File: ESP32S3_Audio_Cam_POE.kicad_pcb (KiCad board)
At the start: 4 copper layers, 56 parts, among them J1 USB-C, U1 USBLC6-2SC6, U2 TLV62568DBVR, U3 ESP32-S3R8, Y1 40MHz, Y2 32.768KHz

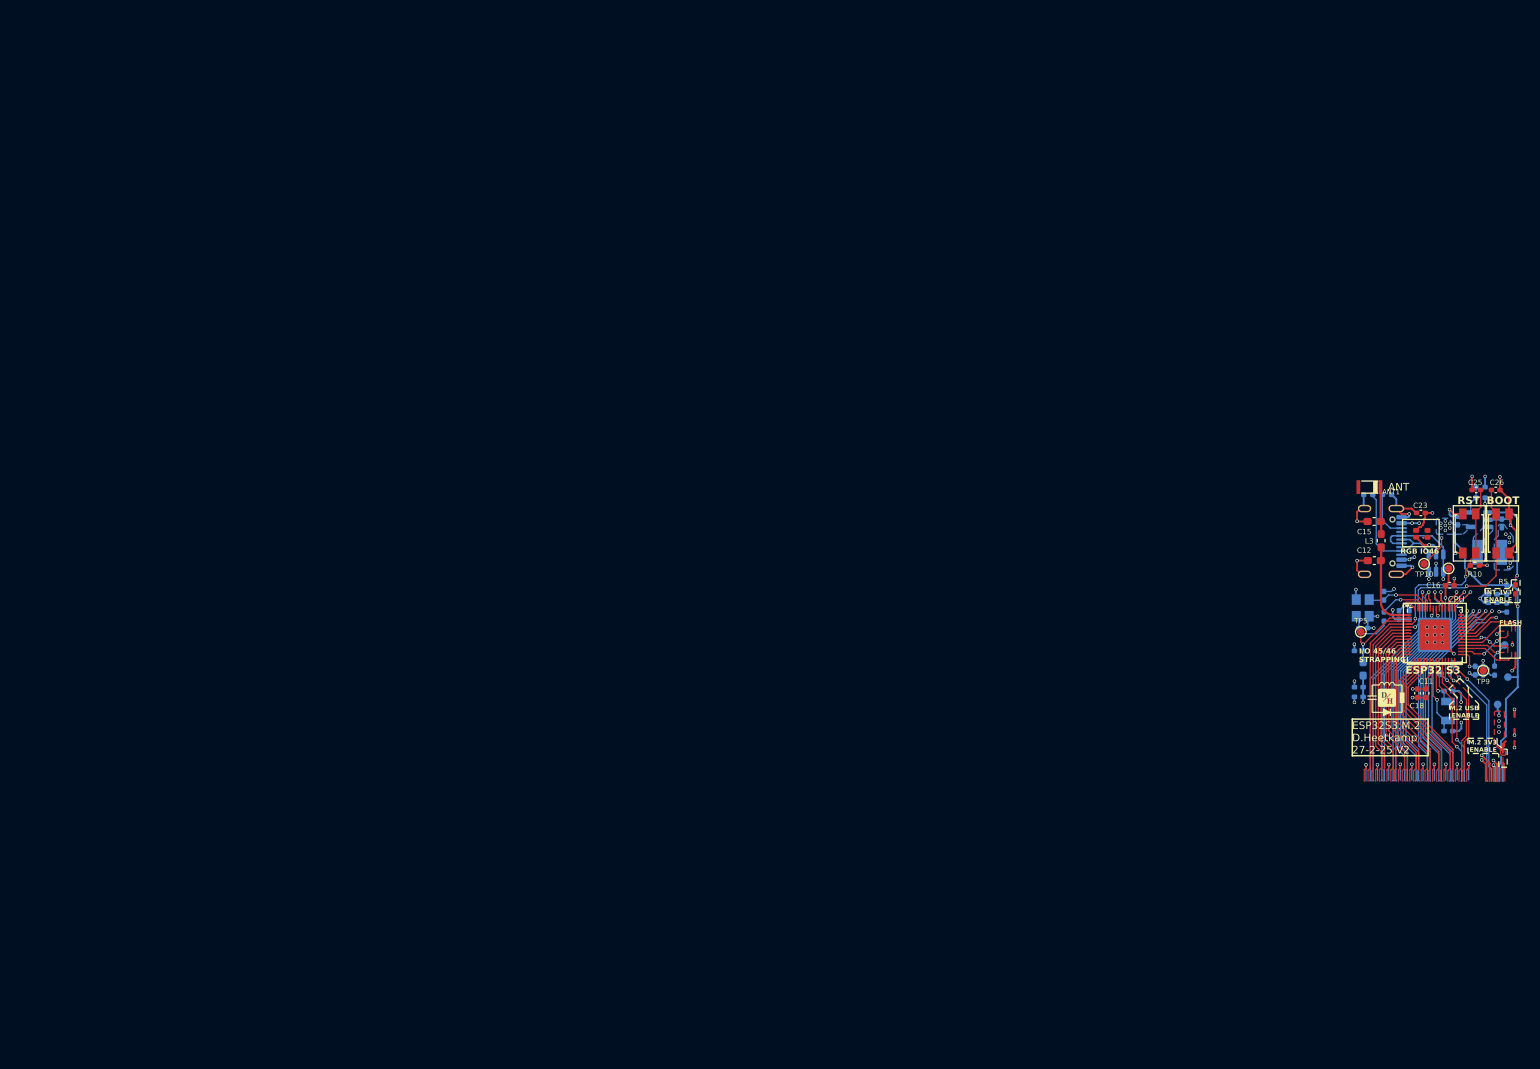
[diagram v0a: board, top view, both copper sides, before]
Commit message: Draft commit, needs routing, schematic is probably mostly OK. Footprints are roughly located.
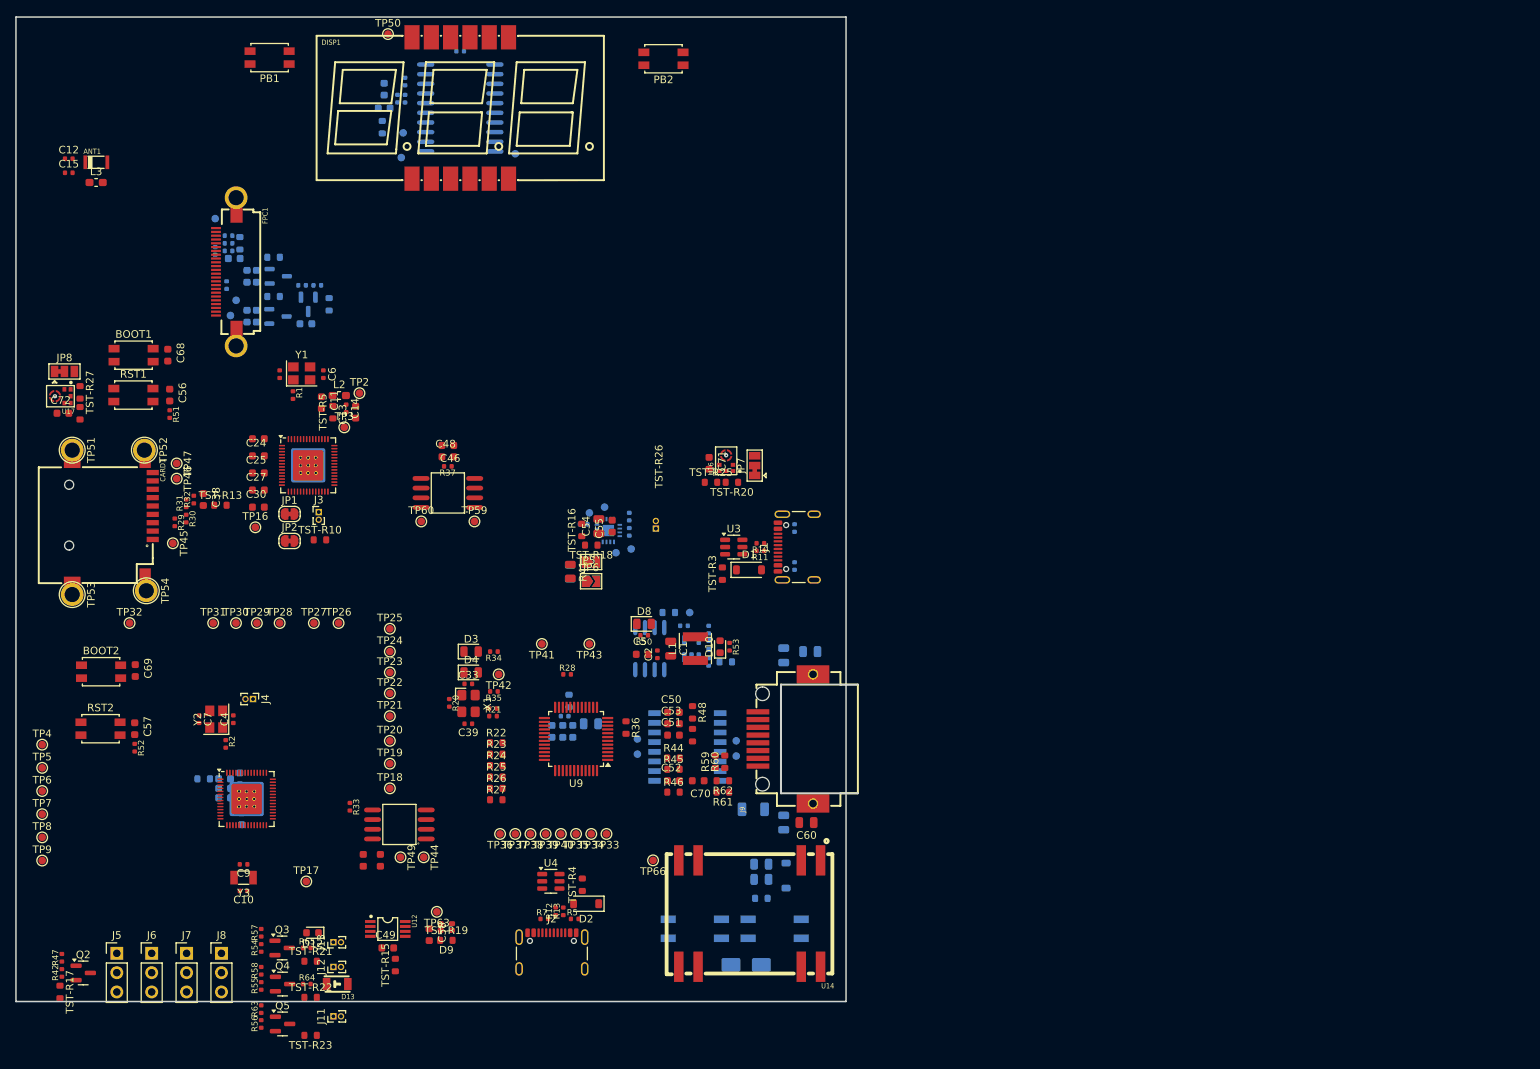
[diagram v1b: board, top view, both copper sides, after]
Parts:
- removed G***: LOGO, LOGO
- removed LED1: WS2812C-2020-V1, PCM_JLCPCB:LED-SMD_4P-L1.6-W1.5_XL-1615RGBC-WS2812B
- removed TP10: TestPoint, TestPoint:TestPoint_Pad_D1.0mm
- added BOOT2: SW_BOOT, Button_Switch_SMD:SW_SPST_EVQP2, F.Cu at (53.4, 117.4)
- added C1: 4.7uF, PCM_JLCPCB:C_0805, F.Cu at (128.4, 114.4)
- added C2: 1nF, PCM_JLCPCB:C_0402, F.Cu at (126.6, 115.2)
- added C27: 100nF, PCM_JLCPCB:C_0603, F.Cu at (74.1, 93.5)
- added C28: 100nF, PCM_JLCPCB:C_0603, B.Cu at (71.7, 131.5)
- added C29: 100nF, PCM_JLCPCB:C_0603, B.Cu at (71.9, 136.8)
- added C3: 10pF, PCM_JLCPCB:C_0402, F.Cu at (76.9, 78.3)
- added C30: 100nF, PCM_JLCPCB:C_0603, F.Cu at (74.1, 95.8)
- added C31: 100nF, PCM_JLCPCB:C_0603, B.Cu at (69.7, 131.5)
- added C32: 100nF, PCM_JLCPCB:C_0603, B.Cu at (69.7, 132.8)
- added C33: 10pF, PCM_JLCPCB:C_0402, F.Cu at (101.8, 119.0)
- added C34: 10pF, PCM_JLCPCB:C_0402, F.Cu at (105.0, 122.3)
- added C35: 100nF, PCM_JLCPCB:C_0603, B.Cu at (114.2, 125.3)
- added C36: 10uF, PCM_JLCPCB:C_0805, B.Cu at (117.9, 124.3)
- added C37: 100nF, PCM_JLCPCB:C_0603, B.Cu at (112.8, 125.3)
- added C38: 100nF, PCM_JLCPCB:C_0603, F.Cu at (66.9, 94.8)
- added C39: 10nF, PCM_JLCPCB:C_0402, F.Cu at (101.8, 124.3)
- added C4: 10pF, PCM_JLCPCB:C_0402, F.Cu at (70.8, 123.7)
- added C40: 4.7uF, PCM_JLCPCB:C_0603, B.Cu at (115.5, 125.3)
- added C41: 100nF, PCM_JLCPCB:C_0603, F.Cu at (90.2, 142.3)
- added C42: 1uF, PCM_JLCPCB:C_0603, F.Cu at (87.9, 142.3)
- added C43: 1uF, PCM_JLCPCB:C_0603, B.Cu at (90.7, 40.8)
- added C44: 100nF, PCM_JLCPCB:C_0603, B.Cu at (90.7, 43.3)
- added C45: 100pF, PCM_JLCPCB:C_0402, B.Cu at (100.7, 35.8)
- added C46: 100nF, PCM_JLCPCB:C_0603, F.Cu at (99.1, 87.7)
- added C47: 100pF, PCM_JLCPCB:C_0402, B.Cu at (93.4, 39.8)
- added C48: 1uF, PCM_JLCPCB:C_0603, F.Cu at (99.1, 89.2)
- added C49: 100nF, PCM_JLCPCB:C_0603, F.Cu at (91.2, 153.8)
- added C5: 100nF, PCM_JLCPCB:C_0603, F.Cu at (124.6, 115.2)
- added C50: 6.8nF, PCM_JLCPCB:C_0603, F.Cu at (128.8, 122.8)
- added C51: 6.8nF, PCM_JLCPCB:C_0603, F.Cu at (128.8, 125.8)
- added C52: 220nF, PCM_JLCPCB:C_0603, F.Cu at (128.8, 131.8)
- added C53: 220nF, PCM_JLCPCB:C_0603, F.Cu at (128.8, 124.3)
- added C54: 10uF, PCM_JLCPCB:C_0805, F.Cu at (118.9, 98.3)
- added C55: 100nF, PCM_JLCPCB:C_0603, F.Cu at (120.7, 98.3)
- added C56: 100nF, PCM_JLCPCB:C_0603, F.Cu at (62.5, 81.0)
- added C57: 100nF, PCM_JLCPCB:C_0603, F.Cu at (57.9, 124.9)
- added C58: 100nF, PCM_JLCPCB:C_0603, F.Cu at (96.6, 152.0)
- added C59: 100nF, PCM_JLCPCB:C_0805, B.Cu at (143.3, 137.3)
- added C60: 100nF, PCM_JLCPCB:C_0805, F.Cu at (146.3, 137.3)
- added C61: 10uF, PCM_JLCPCB:C_0805, B.Cu at (140.3, 144.8)
- added C62: 100nF, PCM_JLCPCB:C_0805, B.Cu at (146.8, 114.8)
- added C63: 100nF, PCM_JLCPCB:C_0805, B.Cu at (143.3, 115.3)
- added C64: 22uF, PCM_JLCPCB:C_0805, B.Cu at (140.3, 142.8)
- added C65: 1nF, PCM_JLCPCB:C_1206, B.Cu at (139.3, 135.5)
- added C66: 220pF, PCM_JLCPCB:C_0402, B.Cu at (122.9, 99.0)
- added C67: 220pF, PCM_JLCPCB:C_0402, B.Cu at (122.9, 97.0)
- added C68: 100nF, PCM_JLCPCB:C_0603, F.Cu at (62.2, 75.8)
- added C69: 100nF, PCM_JLCPCB:C_0603, F.Cu at (57.9, 117.3)
- added C70: 100nF, PCM_JLCPCB:C_0603, F.Cu at (132.0, 131.8)
- added C71: 100nF, PCM_JLCPCB:C_0603, F.Cu at (133.4, 90.0)
- added C72: 100nF, PCM_JLCPCB:C_0603, F.Cu at (48.4, 83.4)
- added CARD1: TF PUSH, JLCPCB:TF-PUSH-SD-CARD_C393941, F.Cu at (54.9, 97.8)
- added D10: Red, PCM_JLCPCB:D_0603, F.Cu at (134.9, 114.2)
- added D11: 1N4148W, PCM_JLCPCB:D_SOD-123, B.Cu at (143.6, 144.3)
- added D12: White, PCM_JLCPCB:D_0603, F.Cu at (81.3, 151.8)
- added D13: IR, JLCPCB:IR-LED_C131280, F.Cu at (84.5, 158.5)
- added D3: Yellow, PCM_JLCPCB:D_0805, F.Cu at (102.1, 114.8)
- added D4: Green, PCM_JLCPCB:D_0805, F.Cu at (102.1, 117.5)
- added D5: MB6S, JLCPCB:MB6S-C82584, B.Cu at (131.6, 151.3)
- added D6: MB6S, JLCPCB:MB6S-C82584, B.Cu at (142.1, 151.3)
- added D7: SMAJ58A, PCM_JLCPCB:D_SMA, B.Cu at (138.3, 156.0)
- added D8: Green, PCM_JLCPCB:D_0805, F.Cu at (124.9, 111.2)
- added D9: WS2812B, PCM_JLCPCB:LED-SMD_4P-L1.6-W1.5_XL-1615RGBC-WS2812B, F.Cu at (98.9, 151.0)
- added DISP1: SLS0563DRA1GD, JLCPCB:3x7-seg_LED-RED_C2913084, F.Cu at (100.7, 43.3)
- added FPC1: AFC01-S24FCC-00, JLCPCB:OV2640_connector_AFC01-S24FCC-00, F.Cu at (69.9, 64.8)
- added J10: Conn_01x02, Connector_PinHeader_1.00mm:PinHeader_1x02_P1.00mm_Vertical, B.Cu at (126.4, 98.6)
- added J11: Conn_01x02, Connector_PinHeader_1.00mm:PinHeader_1x02_P1.00mm_Vertical, F.Cu at (84.0, 162.8)
- added J12: Conn_01x02, Connector_PinHeader_1.00mm:PinHeader_1x02_P1.00mm_Vertical, F.Cu at (84.0, 156.3)
- added J13: Conn_01x02, Connector_PinHeader_1.00mm:PinHeader_1x02_P1.00mm_Vertical, F.Cu at (84.0, 153.0)
- added J2: USB-C, Connector_USB:USB_C_Receptacle_GCT_USB4105-xx-A_16P_TopMnt_Horizontal, F.Cu at (112.8, 155.5)
- added J3: Conn_01x02, Connector_PinHeader_1.00mm:PinHeader_1x02_P1.00mm_Vertical, F.Cu at (82.1, 96.4)
- added J4: Conn_01x02, Connector_PinHeader_1.00mm:PinHeader_1x02_P1.00mm_Vertical, F.Cu at (73.4, 121.0)
- added J5: Conn_01x03, Connector_PinHeader_2.54mm:PinHeader_1x03_P2.54mm_Vertical, F.Cu at (55.5, 154.5)
- added J6: Conn_01x03, Connector_PinHeader_2.54mm:PinHeader_1x03_P2.54mm_Vertical, F.Cu at (60.1, 154.5)
- added J7: Conn_01x03, Connector_PinHeader_2.54mm:PinHeader_1x03_P2.54mm_Vertical, F.Cu at (64.7, 154.5)
- added J8: Conn_01x03, Connector_PinHeader_2.54mm:PinHeader_1x03_P2.54mm_Vertical, F.Cu at (69.3, 154.5)
- added J9: HC-RJ45-055-4_8P8C_Shielded, JLCPCB:HC-RJ45-055-4_C3000211, F.Cu at (143.5, 126.3)
- added JP1: Jumper_2_Small_Bridged, Jumper:SolderJumper-2_P1.3mm_Bridged_RoundedPad1.0x1.5mm, F.Cu at (78.2, 96.7)
- added JP2: Jumper_2_Small_Bridged, Jumper:SolderJumper-2_P1.3mm_Bridged_RoundedPad1.0x1.5mm, F.Cu at (78.2, 100.2)
- added JP3: SolderJumper_2_Open, Jumper:SolderJumper-2_P1.3mm_Open_TrianglePad1.0x1.5mm, B.Cu at (117.9, 105.5)
- added JP4: SolderJumper_2_Open, Jumper:SolderJumper-2_P1.3mm_Open_TrianglePad1.0x1.5mm, B.Cu at (117.9, 103.0)
- added JP5: SolderJumper_2_Open, Jumper:SolderJumper-2_P1.3mm_Open_TrianglePad1.0x1.5mm, F.Cu at (117.9, 103.0)
- added JP6: SolderJumper_2_Open, Jumper:SolderJumper-2_P1.3mm_Open_TrianglePad1.0x1.5mm, F.Cu at (117.9, 105.5)
- added JP7: SolderJumper_3_Bridged12, Jumper:SolderJumper-3_P1.3mm_Bridged12_Pad1.0x1.5mm, F.Cu at (139.4, 90.3)
- added JP8: SolderJumper_3_Bridged12, Jumper:SolderJumper-3_P1.3mm_Bridged12_Pad1.0x1.5mm, F.Cu at (48.6, 77.9)
- added L4: 3.9nH,300mA, PCM_JLCPCB:L_0402, B.Cu at (114.4, 123.3)
- added PB1: SW_RST, Button_Switch_SMD:SW_SPST_EVQP2, F.Cu at (75.6, 36.6)
- added PB2: SW_RST, Button_Switch_SMD:SW_SPST_EVQP2, F.Cu at (127.4, 36.8)
- added Q1: AO3401A, PCM_JLCPCB:Q_SOT-23, B.Cu at (80.7, 69.1)
- added Q2: AO3401A, PCM_JLCPCB:Q_SOT-23, F.Cu at (51.1, 157.1)
- added Q3: AO3401A, PCM_JLCPCB:Q_SOT-23, F.Cu at (77.3, 153.8)
- added Q4: AO3401A, PCM_JLCPCB:Q_SOT-23, F.Cu at (77.3, 158.5)
- added Q5: AO3401A, PCM_JLCPCB:Q_SOT-23, F.Cu at (77.3, 163.8)
- added R13: 33Ω, PCM_JLCPCB:R_0402, F.Cu at (114.3, 149.0)
- added R14: 10MΩ, PCM_JLCPCB:R_0402, B.Cu at (81.9, 66.6)
- added R15: 1MΩ, PCM_JLCPCB:R_0402, B.Cu at (79.9, 66.6)
- added R16: 10kΩ, PCM_JLCPCB:R_0402, B.Cu at (70.2, 60.1)
- added R17: 10kΩ, PCM_JLCPCB:R_0402, B.Cu at (70.2, 61.1)
- added R18: 10kΩ, PCM_JLCPCB:R_0402, B.Cu at (70.2, 62.1)
- added R19: 10kΩ, PCM_JLCPCB:R_0402, B.Cu at (68.5, 62.1)
- added R20: 1MΩ, PCM_JLCPCB:R_0402, F.Cu at (99.3, 121.5)
- added R21: 0Ω, PCM_JLCPCB:R_0402, F.Cu at (105.0, 123.3)
- added R22: 20Ω, PCM_JLCPCB:R_0603, F.Cu at (105.4, 126.8)
- added R23: 20Ω, PCM_JLCPCB:R_0603, F.Cu at (105.4, 128.3)
- added R24: 20Ω, PCM_JLCPCB:R_0603, F.Cu at (105.4, 129.8)
- added R25: 20Ω, PCM_JLCPCB:R_0603, F.Cu at (105.4, 131.3)
- added R26: 20Ω, PCM_JLCPCB:R_0603, F.Cu at (105.4, 132.8)
- added R27: 20Ω, PCM_JLCPCB:R_0603, F.Cu at (105.4, 134.3)
- added R28: 10kΩ, PCM_JLCPCB:R_0402, F.Cu at (114.8, 117.8)
- added R29: 10kΩ, PCM_JLCPCB:R_0402, F.Cu at (63.1, 97.8)
- added R3: 22Ω, PCM_JLCPCB:R_0402, B.Cu at (130.1, 111.4)
- added R30: 10kΩ, PCM_JLCPCB:R_0402, F.Cu at (64.6, 97.3)
- added R31: 10kΩ, PCM_JLCPCB:R_0402, F.Cu at (64.6, 95.3)
- added R32: 10kΩ, PCM_JLCPCB:R_0402, F.Cu at (65.6, 94.8)
- added R33: 100kΩ, PCM_JLCPCB:R_0402, F.Cu at (86.2, 135.2)
- added R34: 680Ω, PCM_JLCPCB:R_0402, F.Cu at (105.1, 114.8)
- added R35: 680Ω, PCM_JLCPCB:R_0402, F.Cu at (105.1, 120.0)
- added R36: 12kΩ, PCM_JLCPCB:R_0603, F.Cu at (122.5, 124.8)
- added R37: 100kΩ, PCM_JLCPCB:R_0402, F.Cu at (99.1, 90.4)
- added R38: 10kΩ, PCM_JLCPCB:R_0402, B.Cu at (92.4, 42.0)
- added R39: 10kΩ, PCM_JLCPCB:R_0402, B.Cu at (93.4, 42.0)
- added R4: 5.1kΩ, PCM_JLCPCB:R_0402, B.Cu at (144.7, 98.5)
- added R40: 100kΩ, PCM_JLCPCB:R_0805, B.Cu at (115.2, 104.3)
- added R41: 100kΩ, PCM_JLCPCB:R_0805, F.Cu at (115.2, 104.3)
- added R42: 10MΩ, PCM_JLCPCB:R_0402, F.Cu at (48.3, 157.1)
- added R43: 1MΩ, PCM_JLCPCB:R_0402, B.Cu at (116.9, 98.0)
- added R44: 47Ω, PCM_JLCPCB:R_0603, F.Cu at (128.8, 128.8)
- added R45: 47Ω, PCM_JLCPCB:R_0603, F.Cu at (128.8, 130.3)
- added R46: 47Ω, PCM_JLCPCB:R_0603, F.Cu at (128.8, 133.3)
- added R47: 1MΩ, PCM_JLCPCB:R_0402, F.Cu at (48.3, 155.1)
- added R48: 82Ω, PCM_JLCPCB:R_0603, F.Cu at (131.3, 122.8)
- added R49: 82Ω, PCM_JLCPCB:R_0603, F.Cu at (131.3, 125.8)
- added R50: 10kΩ, PCM_JLCPCB:R_0402, F.Cu at (124.9, 112.7)
- added R51: 10kΩ, PCM_JLCPCB:R_0402, F.Cu at (62.5, 83.5)
- added R52: 10kΩ, PCM_JLCPCB:R_0402, F.Cu at (57.9, 127.4)
- added R53: 10kΩ, PCM_JLCPCB:R_0402, F.Cu at (136.1, 114.2)
- added R54: 10MΩ, PCM_JLCPCB:R_0402, F.Cu at (74.5, 153.8)
- added R55: 10MΩ, PCM_JLCPCB:R_0402, F.Cu at (74.5, 158.8)
- added R56: 10MΩ, PCM_JLCPCB:R_0402, F.Cu at (74.5, 163.8)
- added R57: 1MΩ, PCM_JLCPCB:R_0402, F.Cu at (74.5, 151.8)
- added R58: 1MΩ, PCM_JLCPCB:R_0402, F.Cu at (74.5, 156.8)
- added R59: 75Ω, PCM_JLCPCB:R_0603, F.Cu at (134.3, 129.3)
- added R60: 75Ω, PCM_JLCPCB:R_0603, F.Cu at (135.5, 129.3)
- added R61: 75Ω, PCM_JLCPCB:R_0603, F.Cu at (135.3, 133.3)
- added R62: 75Ω, PCM_JLCPCB:R_0603, F.Cu at (135.3, 131.8)
- added R63: 1MΩ, PCM_JLCPCB:R_0402, F.Cu at (74.5, 161.8)
- added R64: 10kΩ, PCM_JLCPCB:R_0402, F.Cu at (80.5, 158.5)
- added R65: 10kΩ, PCM_JLCPCB:R_0402, F.Cu at (80.5, 153.8)
- added RST2: SW_RST, Button_Switch_SMD:SW_SPST_EVQP2, F.Cu at (53.4, 124.9)
- added T1: H1102NLT, JLCPCB:H1102NLT_C18584, B.Cu at (130.6, 127.3)
- added TP11: TestPoint, TestPoint:TestPoint_Pad_D1.0mm, B.Cu at (68.5, 57.8)
- added TP12: TestPoint, TestPoint:TestPoint_Pad_D1.0mm, B.Cu at (71.2, 68.6)
- added TP13: TestPoint, TestPoint:TestPoint_Pad_D1.0mm, B.Cu at (70.5, 70.6)
- added TP14: TestPoint, TestPoint:TestPoint_Plated_Hole_D2.0mm, B.Cu at (71.2, 55.1)
- added TP15: TestPoint, TestPoint:TestPoint_Plated_Hole_D2.0mm, B.Cu at (71.2, 74.6)
- added TP16: TestPoint, TestPoint:TestPoint_Pad_D1.0mm, F.Cu at (73.7, 98.4)
- added TP17: TestPoint, TestPoint:TestPoint_Pad_D1.0mm, F.Cu at (80.4, 145.0)
- added TP18: TestPoint, TestPoint:TestPoint_Pad_D1.0mm, F.Cu at (91.4, 132.8)
- added TP19: TestPoint, TestPoint:TestPoint_Pad_D1.0mm, F.Cu at (91.4, 129.5)
- added TP20: TestPoint, TestPoint:TestPoint_Pad_D1.0mm, F.Cu at (91.4, 126.5)
- added TP21: TestPoint, TestPoint:TestPoint_Pad_D1.0mm, F.Cu at (91.4, 123.3)
- added TP22: TestPoint, TestPoint:TestPoint_Pad_D1.0mm, F.Cu at (91.4, 120.3)
- added TP23: TestPoint, TestPoint:TestPoint_Pad_D1.0mm, F.Cu at (91.4, 117.5)
- added TP24: TestPoint, TestPoint:TestPoint_Pad_D1.0mm, F.Cu at (91.4, 114.8)
- added TP25: TestPoint, TestPoint:TestPoint_Pad_D1.0mm, F.Cu at (91.4, 111.8)
- added TP26: TestPoint, TestPoint:TestPoint_Pad_D1.0mm, F.Cu at (84.7, 111.0)
- added TP27: TestPoint, TestPoint:TestPoint_Pad_D1.0mm, F.Cu at (81.4, 111.0)
- added TP28: TestPoint, TestPoint:TestPoint_Pad_D1.0mm, F.Cu at (76.9, 111.0)
- added TP29: TestPoint, TestPoint:TestPoint_Pad_D1.0mm, F.Cu at (73.9, 111.0)
- added TP30: TestPoint, TestPoint:TestPoint_Pad_D1.0mm, F.Cu at (71.2, 111.0)
- added TP31: TestPoint, TestPoint:TestPoint_Pad_D1.0mm, F.Cu at (68.2, 111.0)
- added TP32: TestPoint, TestPoint:TestPoint_Pad_D1.0mm, F.Cu at (57.2, 111.0)
- added TP33: TestPoint, TestPoint:TestPoint_Pad_D1.0mm, F.Cu at (119.9, 138.8)
- added TP34: TestPoint, TestPoint:TestPoint_Pad_D1.0mm, F.Cu at (117.9, 138.8)
- added TP35: TestPoint, TestPoint:TestPoint_Pad_D1.0mm, F.Cu at (115.9, 138.8)
- added TP36: TestPoint, TestPoint:TestPoint_Pad_D1.0mm, F.Cu at (105.9, 138.8)
- added TP37: TestPoint, TestPoint:TestPoint_Pad_D1.0mm, F.Cu at (107.9, 138.8)
- added TP38: TestPoint, TestPoint:TestPoint_Pad_D1.0mm, F.Cu at (109.9, 138.8)
- added TP39: TestPoint, TestPoint:TestPoint_Pad_D1.0mm, F.Cu at (111.9, 138.8)
- added TP40: TestPoint, TestPoint:TestPoint_Pad_D1.0mm, F.Cu at (113.9, 138.8)
- added TP41: TestPoint, TestPoint:TestPoint_Pad_D1.0mm, F.Cu at (111.4, 113.8)
- added TP42: TestPoint, TestPoint:TestPoint_Pad_D1.0mm, F.Cu at (105.8, 117.8)
- added TP43: TestPoint, TestPoint:TestPoint_Pad_D1.0mm, F.Cu at (117.7, 113.8)
- added TP44: TestPoint, TestPoint:TestPoint_Pad_D1.0mm, F.Cu at (95.9, 141.9)
- added TP45: TestPoint, TestPoint:TestPoint_Pad_D1.0mm, F.Cu at (62.9, 100.5)
- added TP46: TestPoint, TestPoint:TestPoint_Pad_D1.0mm, F.Cu at (63.4, 92.0)
- added TP47: TestPoint, TestPoint:TestPoint_Pad_D1.0mm, F.Cu at (63.4, 90.0)
- added TP48: TestPoint, TestPoint:TestPoint_Pad_D1.0mm, B.Cu at (107.9, 49.3)
- added TP49: TestPoint, TestPoint:TestPoint_Pad_D1.0mm, F.Cu at (92.8, 141.9)
- added TP50: TestPoint, TestPoint:TestPoint_Pad_D1.0mm, F.Cu at (91.2, 33.5)
- added TP51: TestPoint, TestPoint:TestPoint_Plated_Hole_D2.0mm, F.Cu at (49.6, 88.3)
- added TP52: TestPoint, TestPoint:TestPoint_Plated_Hole_D2.0mm, F.Cu at (59.1, 88.3)
- added TP53: TestPoint, TestPoint:TestPoint_Plated_Hole_D2.0mm, F.Cu at (49.6, 107.3)
- added TP54: TestPoint, TestPoint:TestPoint_Plated_Hole_D2.0mm, F.Cu at (59.4, 106.8)
- added TP55: TestPoint, TestPoint:TestPoint_Pad_D1.0mm, B.Cu at (137.0, 126.5)
- added TP56: TestPoint, TestPoint:TestPoint_Pad_D1.0mm, B.Cu at (137.0, 128.5)
- added TP57: TestPoint, TestPoint:TestPoint_Pad_D1.0mm, B.Cu at (93.2, 46.5)
- added TP58: TestPoint, TestPoint:TestPoint_Pad_D1.0mm, B.Cu at (92.9, 49.8)
- added TP59: TestPoint, TestPoint:TestPoint_Pad_D1.0mm, F.Cu at (102.6, 97.7)
- added TP6: TestPoint, TestPoint:TestPoint_Pad_D1.0mm, F.Cu at (45.7, 133.1)
- added TP60: TestPoint, TestPoint:TestPoint_Pad_D1.0mm, F.Cu at (95.6, 97.7)
- added TP61: TestPoint, TestPoint:TestPoint_Pad_D1.0mm, B.Cu at (124.0, 126.3)
- added TP62: TestPoint, TestPoint:TestPoint_Pad_D1.0mm, B.Cu at (124.0, 128.3)
- added TP63: TestPoint, TestPoint:TestPoint_Pad_D1.0mm, F.Cu at (97.6, 149.0)
- added TP64: TestPoint, TestPoint:TestPoint_Pad_D1.0mm, B.Cu at (117.7, 96.5)
- added TP65: TestPoint, TestPoint:TestPoint_Pad_D1.0mm, B.Cu at (119.7, 95.8)
- added TP66: TestPoint, TestPoint:TestPoint_Pad_D1.0mm, F.Cu at (126.1, 142.3)
- added TP67: TestPoint, TestPoint:TestPoint_Pad_D1.0mm, B.Cu at (121.2, 101.8)
- added TP68: TestPoint, TestPoint:TestPoint_Pad_D1.0mm, B.Cu at (123.2, 101.3)
- added TST-R1: 0Ω, PCM_JLCPCB:R_0603, B.Cu at (128.1, 109.7)
- added TST-R10: 0Ω, PCM_JLCPCB:R_0603, F.Cu at (82.2, 100.1)
- added TST-R11: 0Ω, PCM_JLCPCB:R_0603, B.Cu at (66.9, 131.5)
- added TST-R12: 0Ω, PCM_JLCPCB:R_0603, B.Cu at (115.0, 121.3)
- added TST-R13: 0Ω, PCM_JLCPCB:R_0603, F.Cu at (69.1, 95.5)
- added TST-R14: 0Ω, PCM_JLCPCB:R_0603, B.Cu at (90.4, 45.8)
- added TST-R15: 0Ω, PCM_JLCPCB:R_0603, F.Cu at (92.2, 156.0)
- added TST-R16: 0Ω, PCM_JLCPCB:R_0603, F.Cu at (116.7, 98.8)
- added TST-R17: 0Ω, PCM_JLCPCB:R_0603, F.Cu at (48.0, 159.6)
- added TST-R18: 0Ω, PCM_JLCPCB:R_0603, F.Cu at (117.9, 100.8)
- added TST-R19: 0Ω, PCM_JLCPCB:R_0603, F.Cu at (98.9, 152.8)
- added TST-R2: 0Ω, PCM_JLCPCB:R_0603, B.Cu at (135.6, 116.2)
- added TST-R20: 0Ω, PCM_JLCPCB:R_0603, F.Cu at (136.4, 92.5)
- added TST-R21: 0Ω, PCM_JLCPCB:R_0603, F.Cu at (81.0, 155.5)
- added TST-R22: 0Ω, PCM_JLCPCB:R_0603, F.Cu at (81.0, 160.3)
- added TST-R23: 0Ω, PCM_JLCPCB:R_0603, F.Cu at (81.0, 165.3)
- added TST-R24: 0Ω, PCM_JLCPCB:R_0603, B.Cu at (140.3, 147.3)
- added TST-R25: 0Ω, PCM_JLCPCB:R_0603, F.Cu at (133.7, 92.5)
- added TST-R26: 0Ω, PCM_JLCPCB:R_0603, F.Cu at (50.7, 83.4)
- added TST-R27: 0Ω, PCM_JLCPCB:R_0603, F.Cu at (50.7, 80.7)
- added TST-R3: 0Ω, PCM_JLCPCB:R_0603, F.Cu at (135.2, 104.5)
- added TST-R4: 0Ω, PCM_JLCPCB:R_0603, F.Cu at (116.8, 145.5)
- added TST-R5: 0Ω, PCM_JLCPCB:R_0603, F.Cu at (83.9, 83.3)
- added TST-R6: 0Ω, PCM_JLCPCB:R_0603, B.Cu at (83.4, 69.1)
- added TST-R7: 0Ω, PCM_JLCPCB:R_0603, B.Cu at (71.7, 61.1)
- added TST-R8: 0Ω, PCM_JLCPCB:R_0603, B.Cu at (76.1, 62.9)
- added TST-R9: 0Ω, PCM_JLCPCB:R_0603, B.Cu at (76.1, 68.1)
- added U10: W25Q128, PCM_JLCPCB:SOIC-8_L5.3-W5.3-P1.27-LS8.0-BL, F.Cu at (92.7, 137.5)
- added U11: TM1637, JLCPCB:digital tube drivers_c2962580, B.Cu at (100.7, 43.3)
- added U12: DS18B20U(UMW), JLCPCB:DS18B20_C695836, F.Cu at (91.2, 151.3)
- added U13: W25Q128, PCM_JLCPCB:SOIC-8_L5.3-W5.3-P1.27-LS8.0-BL, F.Cu at (99.1, 93.9)
- added U14: DP9900M-5V, JLCPCB:DP9900M_C5380106, F.Cu at (138.8, 149.3)
- added U15: MAX98357AETE+T, JLCPCB:MAX98357AETE+T_C910544, B.Cu at (120.2, 98.9)
- added U16: ICS-43434, JLCPCB:ICS-43434_C5656610, F.Cu at (135.7, 89.8)
- added U17: ICS-43434, JLCPCB:ICS-43434_C5656610, F.Cu at (48.2, 81.2)
- added U4: USBLC6-2SC6, Package_TO_SOT_SMD:SOT-23-6, F.Cu at (112.6, 145.0)
- added U5: XC6206-1.5NR, Package_TO_SOT_SMD:SOT-23-3, B.Cu at (76.8, 65.4)
- added U6: XC6206-2.8V, Package_TO_SOT_SMD:SOT-23-3, B.Cu at (76.7, 70.7)
- added U7: ESP32-S3, PCM_JLCPCB:QFN-56-1EP_7x7mm_P0.4mm_EP4x4mm_ThermalVias, F.Cu at (80.7, 90.3)
- added U8: ESP32-S3, PCM_JLCPCB:QFN-56-1EP_7x7mm_P0.4mm_EP4x4mm_ThermalVias, F.Cu at (72.6, 134.2)
- added U9: W5500, Package_QFP:LQFP-48_7x7mm_P0.5mm, F.Cu at (115.9, 126.3)
- added X1: X322525MOB4SI, PCM_JLCPCB:OSC-SMD_4P-L3.2-W2.5-BL, F.Cu at (101.8, 121.6)
- added Y3: 32.768KHz, Crystal:Crystal_SMD_3215-2Pin_3.2x1.5mm, F.Cu at (72.2, 144.5)
- C10: value 10u -> 20pF; footprint Capacitor_SMD:C_0402_1005Metric_Pad0.74x0.62mm_HandSolder -> PCM_JLCPCB:C_0402; moved to F.Cu
- C11, C20: value 1u -> 100nF; footprint Capacitor_SMD:C_0402_1005Metric_Pad0.74x0.62mm_HandSolder -> PCM_JLCPCB:C_0603
- C12, C15: value 3p3 -> 3.3pF; footprint Capacitor_SMD:C_0603_1608Metric_Pad1.08x0.95mm_HandSolder -> PCM_JLCPCB:C_0402
- C13: value 100n -> 100nF; footprint Capacitor_SMD:C_0402_1005Metric_Pad0.74x0.62mm_HandSolder -> PCM_JLCPCB:C_0603; moved to F.Cu
- C14: value 100n -> 10uF; footprint Capacitor_SMD:C_0402_1005Metric_Pad0.74x0.62mm_HandSolder -> PCM_JLCPCB:C_0402; moved to F.Cu
- C16, C18, C26: value 100n -> 1uF; footprint Capacitor_SMD:C_0402_1005Metric_Pad0.74x0.62mm_HandSolder -> PCM_JLCPCB:C_0603; moved to B.Cu
- C17, C23: value 100n -> 1uF; footprint Capacitor_SMD:C_0402_1005Metric_Pad0.74x0.62mm_HandSolder -> PCM_JLCPCB:C_0603
- C19, C21: value 10p -> 100nF; footprint Capacitor_SMD:C_0402_1005Metric_Pad0.74x0.62mm_HandSolder -> PCM_JLCPCB:C_0603
- C22: value 20p -> 15pF; footprint Capacitor_SMD:C_0402_1005Metric_Pad0.74x0.62mm_HandSolder -> PCM_JLCPCB:C_0402
- C24: value 20p -> 100nF; footprint Capacitor_SMD:C_0402_1005Metric_Pad0.74x0.62mm_HandSolder -> PCM_JLCPCB:C_0603; moved to F.Cu
- C25: value 100n -> 100nF; footprint Capacitor_SMD:C_0402_1005Metric_Pad0.74x0.62mm_HandSolder -> PCM_JLCPCB:C_0603
- C6: value 4u7 -> 10pF; footprint Capacitor_SMD:C_0402_1005Metric_Pad0.74x0.62mm_HandSolder -> PCM_JLCPCB:C_0402; moved to F.Cu
- C7: value 10u -> 10pF; footprint Capacitor_SMD:C_0402_1005Metric_Pad0.74x0.62mm_HandSolder -> PCM_JLCPCB:C_0402; moved to F.Cu
- C8: value 100n -> 10uF; footprint Capacitor_SMD:C_0402_1005Metric_Pad0.74x0.62mm_HandSolder -> PCM_JLCPCB:C_0402
- C9: value 100n -> 20pF; footprint Capacitor_SMD:C_0402_1005Metric_Pad0.74x0.62mm_HandSolder -> PCM_JLCPCB:C_0402; moved to F.Cu
- D1, D2: value LED -> 1N4148W; footprint LED_SMD:LED_0402_1005Metric_Pad0.77x0.64mm_HandSolder -> PCM_JLCPCB:D_SOD-123; moved to F.Cu
- J1, L1, L2, TP2, TP3, TP4, TP8, Y1: moved to F.Cu
- R1, R2: value 5k1 -> 22Ω; footprint Resistor_SMD:R_0402_1005Metric_Pad0.72x0.64mm_HandSolder -> PCM_JLCPCB:R_0402; moved to F.Cu
- R10: value 10k -> 33Ω; footprint Resistor_SMD:R_0402_1005Metric_Pad0.72x0.64mm_HandSolder -> PCM_JLCPCB:R_0402
- R11, R12: value 10k -> 33Ω; footprint Resistor_SMD:R_0402_1005Metric_Pad0.72x0.64mm_HandSolder -> PCM_JLCPCB:R_0402; moved to F.Cu
- R5: value 22R -> 5.1kΩ; footprint Resistor_SMD:R_0402_1005Metric_Pad0.72x0.64mm_HandSolder -> PCM_JLCPCB:R_0402
- R6: value 450k -> 5.1kΩ; footprint Resistor_SMD:R_0402_1005Metric_Pad0.72x0.64mm_HandSolder -> PCM_JLCPCB:R_0402
- R7: value 100k -> 5.1kΩ; footprint Resistor_SMD:R_0402_1005Metric_Pad0.72x0.64mm_HandSolder -> PCM_JLCPCB:R_0402; moved to F.Cu
- R8: value 100k -> 450k
- R9: value 22R -> 100kΩ; footprint Resistor_SMD:R_0402_1005Metric_Pad0.72x0.64mm_HandSolder -> PCM_JLCPCB:R_0402
- U1: value USBLC6-2SC6 -> TLV62568DBVR; footprint Package_TO_SOT_SMD:SOT-23-6 -> Package_TO_SOT_SMD:SOT-23-5
- U2: value TLV62568DBVR -> MT9221CT-06BR5; footprint Package_TO_SOT_SMD:SOT-23-5 -> JLCPCB:Current-sensor_MT9221CT-06BR5_C879632
- U3: value ESP32-S3R8 -> USBLC6-2SC6; footprint PCM_JLCPCB:QFN-56-1EP_7x7mm_P0.4mm_EP4x4mm_ThermalVias -> Package_TO_SOT_SMD:SOT-23-6
- Y2: value 32.768KHz -> 40MHz; footprint Crystal:Crystal_SMD_3215-2Pin_3.2x1.5mm -> Crystal:Crystal_SMD_3225-4Pin_3.2x2.5mm; moved to F.Cu
- moved TP8 194.1 mm to (45.7, 139.2)
- moved TP4 191.6 mm to (45.7, 127.0), turned to 0 degrees
- moved TP9 191.2 mm to (45.7, 142.3)
- moved TP7 187.9 mm to (45.7, 136.2)
- moved BOOT1 181.7 mm to (57.7, 75.8), turned to 0 degrees
- moved C12 179.7 mm to (49.2, 49.9), turned to 0 degrees
- moved C15 177.8 mm to (49.2, 51.8), turned to 0 degrees
- moved RST1 176.7 mm to (57.7, 81.0), turned to 0 degrees
- moved L3 175.5 mm to (52.8, 53.1), turned to 0 degrees
- moved TP5 174.4 mm to (45.7, 130.1)
- moved C7 173.3 mm to (66.3, 123.7), turned to -90 degrees
- moved ANT1 172.9 mm to (52.8, 50.4), turned to 0 degrees
- moved C26 172.1 mm to (69.7, 134.0), turned to 180 degrees
- moved C22 171.1 mm to (70.0, 66.6), turned to -90 degrees
- moved C20 169.2 mm to (72.6, 70.7), turned to 90 degrees
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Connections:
- C10 pad 1: +3V3 -> /2OSC32_OUT
- C11 pad 1: +3V3 -> Earth
- C11 pad 2: Earth -> +3V3_RF
- C13 pad 1: +3V3 -> Earth
- C13 pad 2: Earth -> +3V3
- C16 pad 1: +3V3 -> Net-(Q1-D)
- C17 pad 1: VDD_SPI -> Net-(U5-VO)
- C18 pad 1: +3V3 -> Net-(U6-VO)
- C19 pad 1: Net-(C19-Pad1) -> Earth
- C19 pad 2: Earth -> Net-(U5-VO)
- C20 pad 1: VDD_SPI -> Earth
- C20 pad 2: Earth -> Net-(U6-VO)
- C21 pad 1: /OSC_OUT -> Earth
- C21 pad 2: Earth -> /CAM.RST
- C22 pad 1: /OSC32_IN -> Earth
- C22 pad 2: Earth -> /CAM.PCLK
- C23 pad 1: +3V3 -> Earth
- C23 pad 2: Earth -> Net-(U7-VDD3P3_RTC)
- C24 pad 1: /OSC32_OUT -> Net-(U7-VDD3P3_RTC)
- C25 pad 1: /CHIP_PU -> Net-(U7-VDD3P3_RTC)
- C26 pad 1: /CHIP_BOOT -> Earth
- C26 pad 2: Earth -> Net-(U8-VDD3P3_RTC)
- C6 pad 1: VBUS -> /OSC_OUT
- C7 pad 1: +3V3 -> /2OSC_OUT
- C8 pad 1: +3V3_RF -> Net-(C8-Pad1)
- C9 pad 1: +3V3 -> /2OSC32_IN
- D1 pad 1: Earth -> VBUS
- D1 pad 2: Net-(D1-A) -> Net-(D1-Pad2)
- D2 pad 1: Earth -> VBUS
- D2 pad 2: Net-(D2-A) -> Net-(D2-Pad2)
- J1 pad A4: VBUS -> Net-(D1-Pad2)
- J1 pad A9: VBUS -> Net-(D1-Pad2)
- J1 pad B4: VBUS -> Net-(D1-Pad2)
- J1 pad B9: VBUS -> Net-(D1-Pad2)
- L1 pad 1: Net-(U2-SW) -> Net-(U1-SW)
- L1 pad 2: +3V3 -> Net-(C8-Pad1)
- L2 pad 1: +3V3_RF -> Net-(L2-Pad1)
- R1 pad 1: /USB_CC2 -> Net-(C3-Pad1)
- R1 pad 2: Earth -> /OSC_IN
- R10 pad 1: +3V3 -> /USB_PRT_D-
- R10 pad 2: /CHIP_PU -> /USB_D-
- R11 pad 1: VBUS -> /USB_PRT_D+
- R11 pad 2: Net-(D1-A) -> /USB_D+
- R12 pad 1: +3V3 -> /2USB_PRT_D-
- R12 pad 2: Net-(D2-A) -> /2USB_D-
- R2 pad 1: /USB_CC1 -> Net-(C4-Pad1)
- R2 pad 2: Earth -> /2OSC_IN
- R5 pad 1: VBUS -> /2USB_CC2
- R5 pad 2: Net-(U2-EN) -> Earth
- R6 pad 1: +3V3 -> /USB_CC1
- R6 pad 2: Net-(U2-FB) -> Earth
- R7 pad 1: Net-(U2-FB) -> /2USB_CC1
- R8 pad 1: /FLASH_QSPI_nCS -> Net-(C8-Pad1)
- R8 pad 2: VDD_SPI -> Net-(U1-FB)
- R9 pad 1: /OSC_IN -> Net-(U1-FB)
- R9 pad 2: Net-(C19-Pad1) -> Earth
- TP1 pad 1: /USB_D- -> Net-(U1-VIN)
- TP2 pad 1: /USB_D+ -> +3V3
- TP3 pad 1: VBUS -> Net-(L2-Pad1)
- TP4 pad 1: +3V3 -> /2GPIO1
- TP5 pad 1: +3V3_RF -> /2GPIO2
- TP7 pad 1: +3V3 -> /2GPIO7
- TP8 pad 1: /FLASH_QSPI_nCS -> /2GPIO8
- TP9 pad 1: VDD_SPI -> /2GPIO14
- U1 pad 1: /USB_D- -> Net-(U1-EN)
- U1 pad 3: /USB_D+ -> Net-(U1-SW)
- U1 pad 4: /USB_D+ -> Net-(U1-VIN)
- U1 pad 5: VBUS -> Net-(U1-FB)
- U2 pad 1: Net-(U2-EN) -> Vdrive
- U2 pad 2: Earth -> Vdrive
- U2 pad 3: Net-(U2-SW) -> VBUS
- U2 pad 5: Net-(U2-FB) -> Earth
- U3 pad 1: /RF1 -> /USB_D-
- U3 pad 2: +3V3_RF -> Earth
- U3 pad 3: +3V3_RF -> /USB_D+
- U3 pad 4: /CHIP_PU -> /USB_D+
- U3 pad 5: /CHIP_BOOT -> Net-(U3-VBUS)
- U3 pad 6: /GPIO1 -> /USB_D-
- Y1 pad 1: Net-(C19-Pad1) -> Net-(C3-Pad1)
- Y2 pad 1: /OSC32_IN -> Net-(C4-Pad1)
- Y2 pad 2: /OSC32_OUT -> Earth
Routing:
- net Earth: track 143.5 -> 0.00 mm, vias 45 -> 0
- net (no net): track 109.4 -> 0.00 mm, vias 2 -> 0
- net /CHIP_BOOT: track 52.3 -> 0.00 mm, vias 2 -> 0
- net /CHIP_PU: track 49.5 -> 0.00 mm, vias 2 -> 0
- net VBUS: track 49.1 -> 0.00 mm, vias 13 -> 0
- net /SPICLK_N: track 32.8 -> 0.00 mm, vias 1 -> 0
- net /SPICLK_P: track 32.8 -> 0.00 mm, vias 1 -> 0
- net /GPIO38: track 32.6 -> 0.00 mm, vias 1 -> 0
- net /MTCK: track 31.6 -> 0.00 mm, vias 1 -> 0
- net /MTDO: track 31.0 -> 0.00 mm, vias 1 -> 0
- net /GPIO33: track 31.0 -> 0.00 mm, vias 1 -> 0
- net +3V3: track 30.7 -> 0.00 mm, vias 18 -> 0
- net /MTMS: track 30.4 -> 0.00 mm, vias 1 -> 0
- net /GPIO45: track 30.2 -> 0.00 mm, vias 1 -> 0
- net /MTDI: track 30.1 -> 0.00 mm, vias 1 -> 0
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- removed copper zone on B.Cu, net +3V3
- removed copper zone on F.Cu, net +3V3
- removed copper zone on In2.Cu, net +3V3
- removed copper zone on In1.Cu, net Earth
- removed copper zone on B.Cu, net Net-(U2-SW)
- removed copper zone on B.Cu, net VBUS
- removed copper zone on In2.Cu, net VBUS
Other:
- board outline added: 109.2 x 129.5 mm
- board text removed: "ANT"
- board text removed: "BOOT"
- board text removed: "CPU"
- board text removed: "ESP32 S3"
- board text removed: "ESP32S3.M.2 D.Heetkamp 27-2-25 V2"
- board text removed: "FLASH"
- board text removed: "I/O 45/46 STRAPPING"
- board text removed: "I2C(P/U Res)"
- board text removed: "INT 3V3 ENABLE"
- board text removed: "M.2 3V3 ENABLE"
- board text removed: "M.2 USB ENABLE"
- board text removed: "M.2 VBUS ENABLE"
- board text removed: "RGB IO46"
- board text removed: "RST"
- board text removed: "SPICLK(P/D Res)"
- board text removed: "USB"
- board text removed: "VBUS 3V3"
- board text removed: "Y1: 40MHz Y2: 32.8KHz"
